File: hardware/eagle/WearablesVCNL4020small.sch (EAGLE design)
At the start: 11 parts

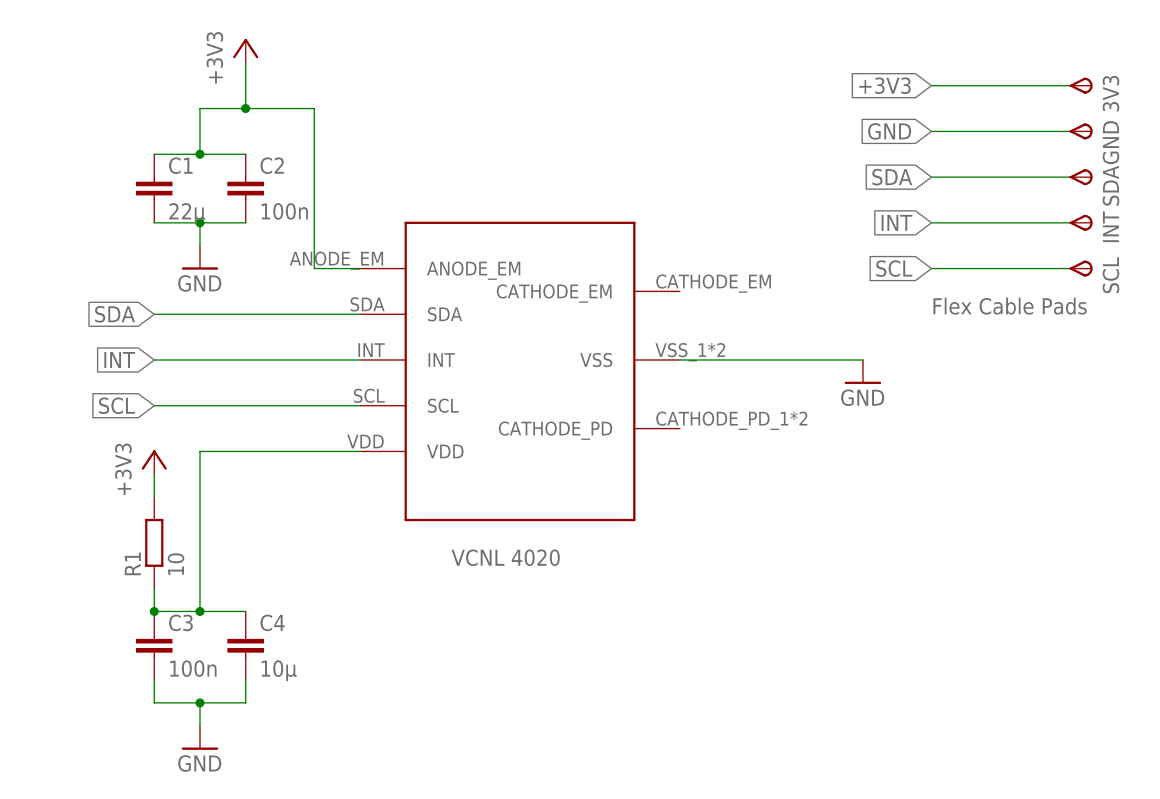
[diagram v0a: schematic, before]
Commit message: updated schematics and board files.
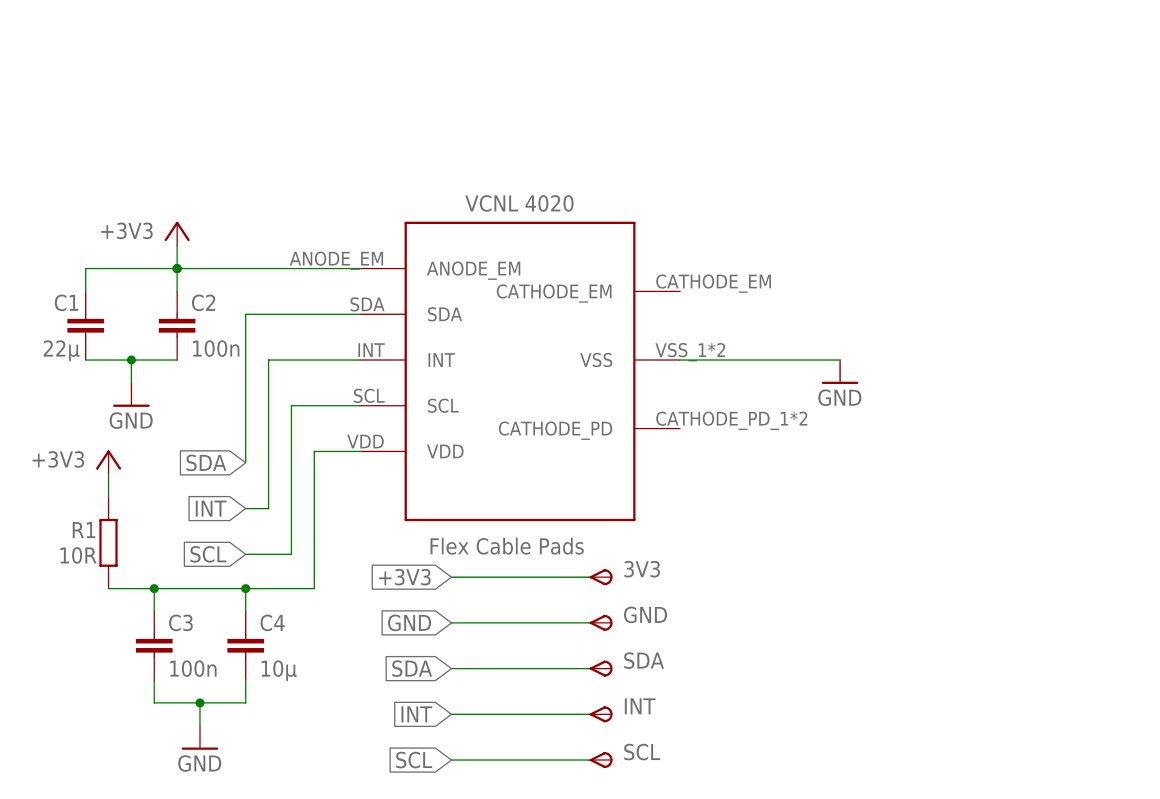
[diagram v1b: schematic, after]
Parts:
- R1: value 10 -> 10R
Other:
- moved on the sheet: 3V3, C1, C2, GND, INT, R1, SCL, SDA
